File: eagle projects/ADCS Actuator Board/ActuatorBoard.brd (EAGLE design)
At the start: 91 x 91 mm, 278 parts, among them J19 TE_1-84953-1, J20 TE_1-84953-1, J21 TE_1-84953-1, U10 DRV10970_MOTOR_DRIVERDRV10970, U12 DRV10970_MOTOR_DRIVERDRV10970, U13 ADS7841E_2K5, U15 TLV9051IDCKR, U19 TLV9051IDCKR, U2 ADS7841E_2K5, U21 TLV9051IDCKR, U23 TLV9051IDCKR, U24 TLV9051IDCKR, U25 ADS7841E_2K5, U26 TLV9051IDCKR, U27 ADS7841E_2K5, U28 TLV9051IDCKR, U29 TLV9051IDCKR, U3 ADS7841E_2K5, U30 TLV9051IDCKR, U31 TLV9051IDCKR, U32 TLV9051IDCKR, U34 TVS991, U35 BD6210F-E2, U38 TVS991, U39 BD6210F-E2, U4 ADS7841E_2K5, U5 TVS991, U6 TLV9051IDCKR, U7 DRV10970_MOTOR_DRIVERDRV10970, U9 BD6210F-E2

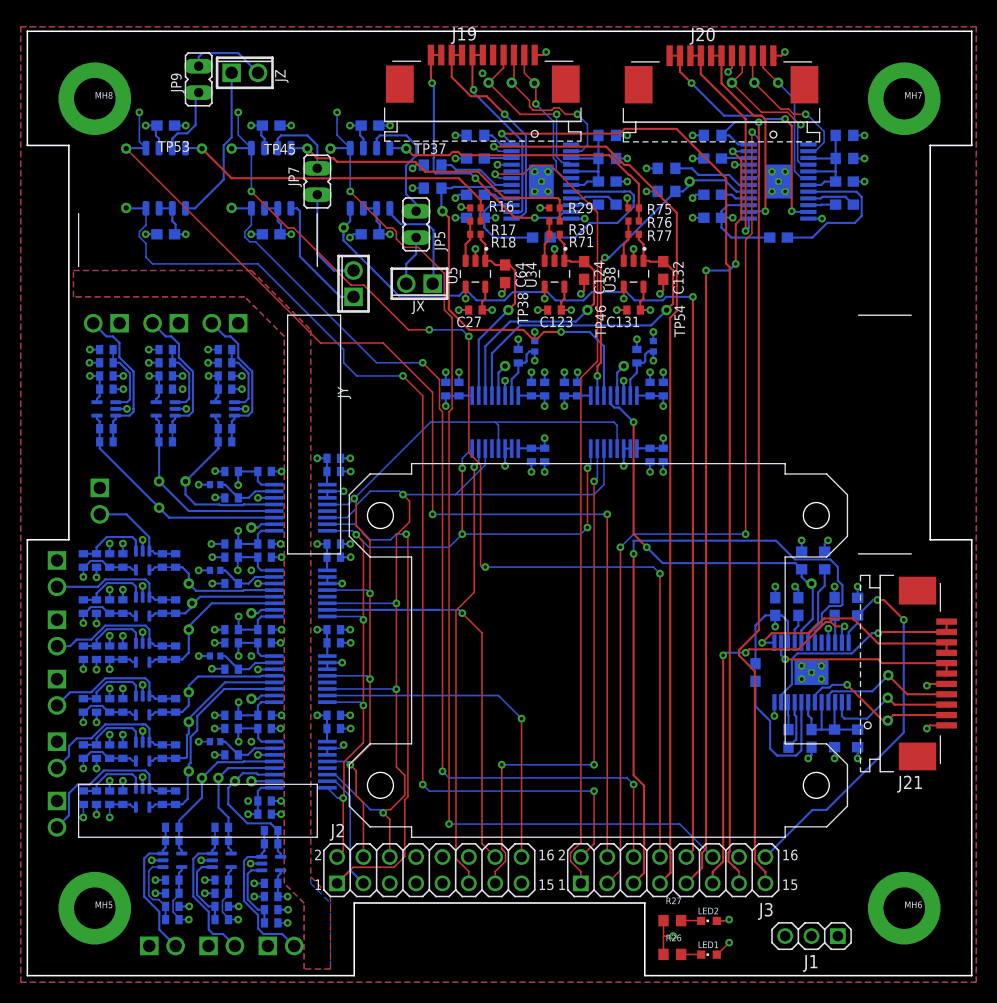
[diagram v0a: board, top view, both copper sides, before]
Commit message: minor layout tweaks
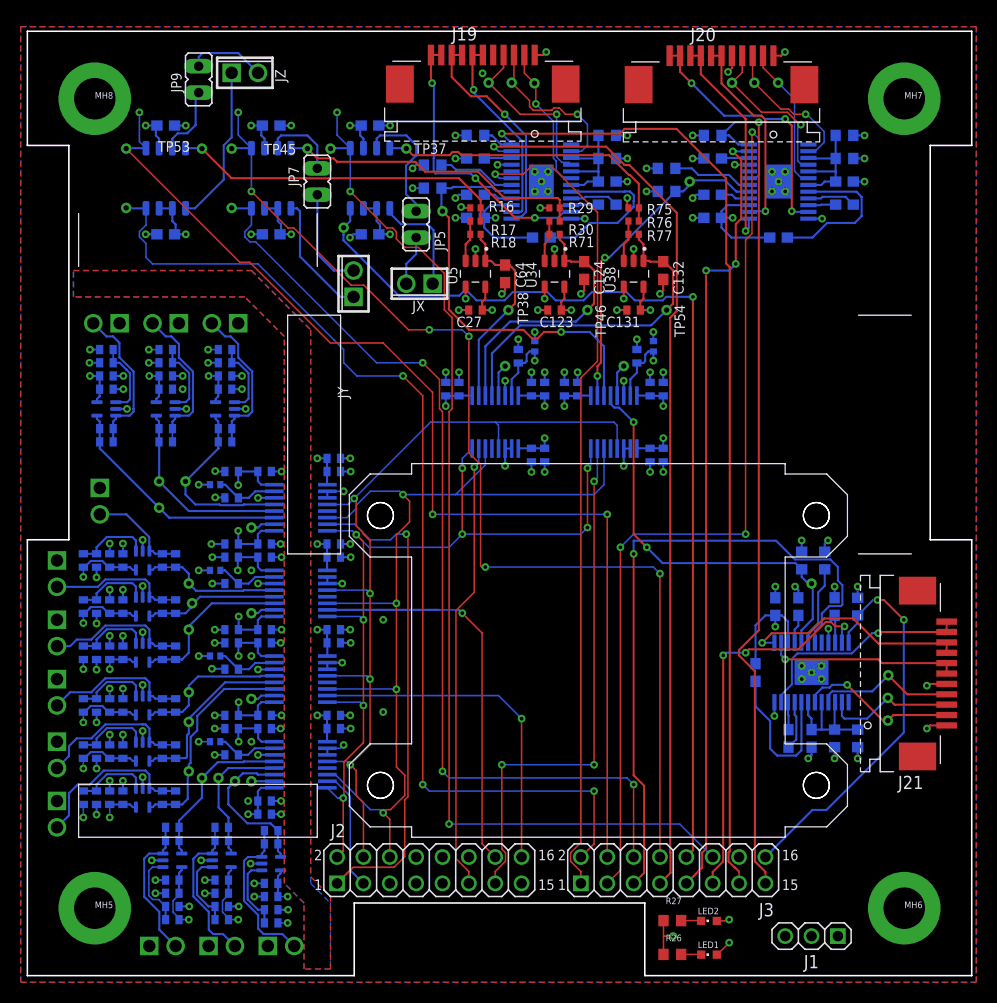
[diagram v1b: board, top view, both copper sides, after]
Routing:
- net GND: vias 170 -> 172
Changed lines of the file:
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@@
 <setting verticaltext="up"/>
 </settings>
-<grid distance="1" unitdist="mil" unit="mil" style="lines" multiple="1" display="yes" altdistance="12.5" altunitdist="mil" altunit="mm"/>
+<grid distance="50" unitdist="mil" unit="mil" style="lines" multiple="1" display="yes" altdistance="12.5" altunitdist="mil" altunit="mil"/>
 <layers>
 <layer number="1" name="Top" color="4" fill="1" visible="yes" active="yes"/>
@@
 </layers>
 <board>
-<fusionsync huburn="a.YnVzaW5lc3M6bXlkYWwyMA" projecturn="a.YnVzaW5lc3M6bXlkYWwyMCMyMDIxMDExNjM3MjQwMzc3Ng" f3durn="urn:adsk.wipprod:dm.lineage:TKW3tc-mS0qsFWWO9AN0Ug" pcbguid="" lastpulledtime="" lastsyncedchangeguid="" latestrevisionid="0074a831-43cd-42bd-b3bd-cc89c6651567" lastsyncedrevisionid="0074a831-43cd-42bd-b3bd-cc89c6651567" lastboardhashguid="857bcac5-dcdf-7e34-be52-16fdd3c31308" lastpushedtime="2021-02-03T02:47:48Z" linktopcb3d="false"/>
+<fusionsync huburn="a.YnVzaW5lc3M6bXlkYWwyMA" projecturn="a.YnVzaW5lc3M6bXlkYWwyMCMyMDIxMDExNjM3MjQwMzc3Ng" f3durn="urn:adsk.wipprod:dm.lineage:TKW3tc-mS0qsFWWO9AN0Ug" pcbguid="" lastpulledtime="2021-02-14T18:09:55Z" lastsyncedchangeguid="" latestrevisionid="c2152030-a1ea-4700-91c3-66171d633219" lastsyncedrevisionid="c2152030-a1ea-4700-91c3-66171d633219" lastboardhashguid="a1286e25-3132-5004-a41b-18cce8fad25a" lastpushedtime="2021-02-14T18:11:04Z" linktopcb3d="true"/>
 <plain>
-<wire x1="0" y1="0" x2="31.5" y2="0" width="0.1524" layer="20" locked="yes"/>
-<wire x1="31.5" y1="0" x2="31.5" y2="7" width="0.1524" layer="20" locked="yes"/>
-<wire x1="31.5" y1="7" x2="59.5" y2="7" width="0.1524" layer="20" locked="yes"/>
-<wire x1="59.5" y1="7" x2="59.5" y2="0" width="0.1524" layer="20" locked="yes"/>
-<wire x1="59.5" y1="0" x2="91" y2="0" width="0.1524" layer="20" locked="yes"/>
-<wire x1="91" y1="0" x2="91" y2="42" width="0.1524" layer="20" locked="yes"/>
-<wire x1="91" y1="42" x2="87" y2="42" width="0.1524" layer="20" locked="yes"/>
-<wire x1="87" y1="42" x2="87" y2="80" width="0.1524" layer="20" locked="yes"/>
-<wire x1="87" y1="80" x2="91" y2="80" width="0.1524" layer="20" locked="yes"/>
-<wire x1="91" y1="80" x2="91" y2="91" width="0.1524" layer="20" locked="yes"/>
-<wire x1="91" y1="91" x2="0" y2="91" width="0.1524" layer="20" locked="yes"/>
-<wire x1="0" y1="91" x2="0" y2="80" width="0.1524" layer="20" locked="yes"/>
-<wire x1="0" y1="80" x2="4" y2="80" width="0.1524" layer="20" locked="yes"/>
-<wire x1="4" y1="80" x2="4" y2="42" width="0.1524" layer="20" locked="yes"/>
-<wire x1="4" y1="42" x2="0" y2="42" width="0.1524" layer="20" locked="yes"/>
-<wire x1="0" y1="42" x2="0" y2="0" width="0.1524" layer="20" locked="yes"/>
 <text x="64.6176" y="16.4719" size="1.016" layer="51" font="vector" rot="R90">ACTUATOR BOARD - REV A</text>
 <text x="65.9511" y="16.4719" size="1.016" layer="151" font="vector" rot="R90">Dalhousie Space Systems Lab</text>
@@
 <rectangle x1="72.6059" y1="66.3067" x2="73.2155" y2="66.3321" locked="yes" layer="203" rot="R180" grouprefs="BOTTOM_LOGO"/>
 <rectangle x1="72.8091" y1="66.3321" x2="73.0631" y2="66.3575" locked="yes" layer="203" rot="R180" grouprefs="BOTTOM_LOGO"/>
+<hole x="34.025" y="44.335" drill="2.5"/>
+<hole x="76.025" y="18.335" drill="2.5"/>
+<hole x="76.025" y="44.335" drill="2.5"/>
+<hole x="34.025" y="18.335" drill="2.5"/>
+<wire x1="0" y1="42" x2="0" y2="0" width="0.1524" layer="20"/>
+<wire x1="0" y1="0" x2="31.5" y2="0" width="0.1524" layer="20"/>
+<wire x1="31.5" y1="0" x2="31.5" y2="7" width="0.1524" layer="20"/>
+<wire x1="31.5" y1="7" x2="59.5" y2="7" width="0.1524" layer="20"/>
+<wire x1="59.5" y1="7" x2="59.5" y2="0" width="0.1524" layer="20"/>
+<wire x1="59.5" y1="0" x2="91" y2="0" width="0.1524" layer="20"/>
+<wire x1="91" y1="0" x2="91" y2="42" width="0.1524" layer="20"/>
+<wire x1="91" y1="42" x2="87" y2="42" width="0.1524" layer="20"/>
+<wire x1="87" y1="42" x2="87" y2="80" width="0.1524" layer="20"/>
+<wire x1="87" y1="80" x2="91" y2="80" width="0.1524" layer="20"/>
+<wire x1="91" y1="80" x2="91" y2="91" width="0.1524" layer="20"/>
+<wire x1="91" y1="91" x2="0" y2="91" width="0.1524" layer="20"/>
+<wire x1="0" y1="91" x2="0" y2="80" width="0.1524" layer="20"/>
+<wire x1="0" y1="80" x2="4" y2="80" width="0.1524" layer="20"/>
+<wire x1="4" y1="80" x2="4" y2="42" width="0.1524" layer="20"/>
+<wire x1="4" y1="42" x2="0" y2="42" width="0.1524" layer="20"/>
 </plain>
 <attributes>
@@
 <attribute name="MF" value="" x="6.985" y="45.72" size="1.778" layer="28" rot="MR270" display="off"/>
 <attribute name="MPN" value="" x="6.985" y="45.72" size="1.778" layer="28" rot="MR270" display="off"/>
-<attribute name="NAME" x="4.572" y="46.609" size="1.016" layer="26" rot="MR270"/>
+<attribute name="NAME" x="10.287" y="47.244" size="1.016" layer="26" rot="MR270"/>
 <attribute name="OC_FARNELL" value="unknown" x="6.985" y="45.72" size="1.778" layer="28" rot="MR270" display="off"/>
 <attribute name="OC_NEWARK" value="unknown" x="6.985" y="45.72" size="1.778" layer="28" rot="MR270" display="off"/>
@@
 <wire x1="11.43" y1="69.215" x2="12.065" y2="68.58" width="0.1524" layer="16"/>
 <wire x1="12.065" y1="68.58" x2="22.225" y2="68.58" width="0.1524" layer="16"/>
-<wire x1="22.225" y1="68.58" x2="30.48" y2="60.325" width="0.1524" layer="16"/>
+<wire x1="22.225" y1="68.58" x2="29.5275" y2="61.2775" width="0.1524" layer="16"/>
+<wire x1="29.5275" y1="61.2775" x2="30.1625" y2="60.6425" width="0.1524" layer="16"/>
+<wire x1="30.1625" y1="60.6425" x2="30.48" y2="60.325" width="0.1524" layer="16"/>
 <wire x1="30.48" y1="60.325" x2="30.48" y2="59.055" width="0.1524" layer="16"/>
 <wire x1="30.48" y1="59.055" x2="31.75" y2="57.785" width="0.1524" layer="16"/>
@@
 <wire x1="39.0525" y1="44.45" x2="39.0525" y2="56.1975" width="0.1524" layer="1"/>
 <wire x1="39.0525" y1="56.1975" x2="34.29" y2="60.96" width="0.1524" layer="1"/>
-<wire x1="34.29" y1="60.96" x2="28.2575" y2="60.96" width="0.1524" layer="1"/>
-<wire x1="28.2575" y1="60.96" x2="9.525" y2="79.6925" width="0.1524" layer="1"/>
+<wire x1="29.21" y1="60.96" x2="34.29" y2="60.96" width="0.1524" layer="1"/>
+<wire x1="9.525" y1="79.6925" x2="20.47875" y2="68.73875" width="0.1524" layer="1"/>
+<wire x1="20.47875" y1="68.73875" x2="21.43125" y2="68.73875" width="0.1524" layer="1"/>
+<wire x1="21.43125" y1="68.73875" x2="29.21" y2="60.96" width="0.1524" layer="1"/>
 </signal>
 <signal name="GND">
@@
 <via x="67.5206" y="87.0821" extent="1-16" drill="0.35"/>
 <via x="43.863940625" y="86.946059375" extent="1-16" drill="0.35"/>
+<via x="34.29" y="34.29" extent="1-16" drill="0.35"/>
+<via x="34.29" y="25.4" extent="1-16" drill="0.35"/>
 </signal>
 <signal name="+5V">
@@
 <wire x1="69.8218" y1="71.50365" x2="69.8218" y2="81.2518" width="0.1524" layer="1"/>
 <wire x1="69.85" y1="81.28" x2="70.53285" y2="80.59715" width="0.1524" layer="16"/>
-<wire x1="70.53285" y1="80.59715" x2="70.53285" y2="77.47" width="0.1524" layer="16"/>
-<wire x1="70.53285" y1="77.47" x2="70.53285" y2="77.1944125" width="0.1524" layer="16"/>
+<wire x1="70.53285" y1="80.59715" x2="70.53285" y2="77.1944125" width="0.1524" layer="16"/>
 <wire x1="70.53285" y1="77.1944125" x2="70.1809375" y2="76.8425" width="0.1524" layer="16"/>
 <wire x1="70.1809375" y1="76.8425" x2="69.5183" y2="76.8425" width="0.1524" layer="16"/>
@@
 <wire x1="43" y1="85.365" x2="42.89" y2="85.475" width="0.2" layer="1"/>
 <wire x1="42.89" y1="85.475" x2="42.89" y2="88.71" width="0.2" layer="1"/>
-<wire x1="47.69665" y1="73.73165" x2="47.69665" y2="80" width="0.2" layer="16"/>
+<wire x1="47.69665" y1="73.73165" x2="47.69665" y2="80.40045" width="0.2" layer="16"/>
 <wire x1="42.89" y1="88.71" x2="43.89" y2="88.71" width="0.2" layer="1"/>
-<wire x1="47.69665" y1="80" x2="47.69665" y2="80.40045" width="0.2" layer="16"/>
 <wire x1="43" y1="85.0971" x2="43" y2="85.365" width="0.2" layer="16"/>
 <wire x1="47.69665" y1="80.40045" x2="43" y2="85.0971" width="0.2" layer="16"/>
@@
 <wire x1="46.0756" y1="11.840325" x2="46.0756" y2="11.019675" width="0.1524" layer="1"/>
 <wire x1="45.085" y1="10.029075" x2="45.085" y2="8.89" width="0.1524" layer="1"/>
-<wire x1="46.0756" y1="11.840325" x2="45.7854625" y2="12.1304625" width="0.1524" layer="1"/>
+<wire x1="46.0756" y1="11.840325" x2="45.72" y2="12.195925" width="0.1524" layer="1"/>
 <wire x1="46.0756" y1="11.019675" x2="45.085" y2="10.029075" width="0.1524" layer="1"/>
 <contactref element="U3" pad="15"/>
@@
 <via x="45.72" y="20.32" extent="1-16" drill="0.35"/>
 <wire x1="45.72" y1="20.32" x2="45.72" y2="12.195925" width="0.1524" layer="1"/>
-<wire x1="45.72" y1="12.195925" x2="45.7854625" y2="12.1304625" width="0.1524" layer="1"/>
 </signal>
 <signal name="!CS!_CUR_SENSE_MAG">
